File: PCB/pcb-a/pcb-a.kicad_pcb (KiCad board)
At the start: 2 copper layers, 89.4 x 42.2 mm, 29 parts, among them J1 Conn_02x05_Counter_Clockwise, J2 Conn_02x04_Counter_Clockwise, Q3 BC337, SW1 config, U1 ESP32-S2-DevKitM, U3 L7805

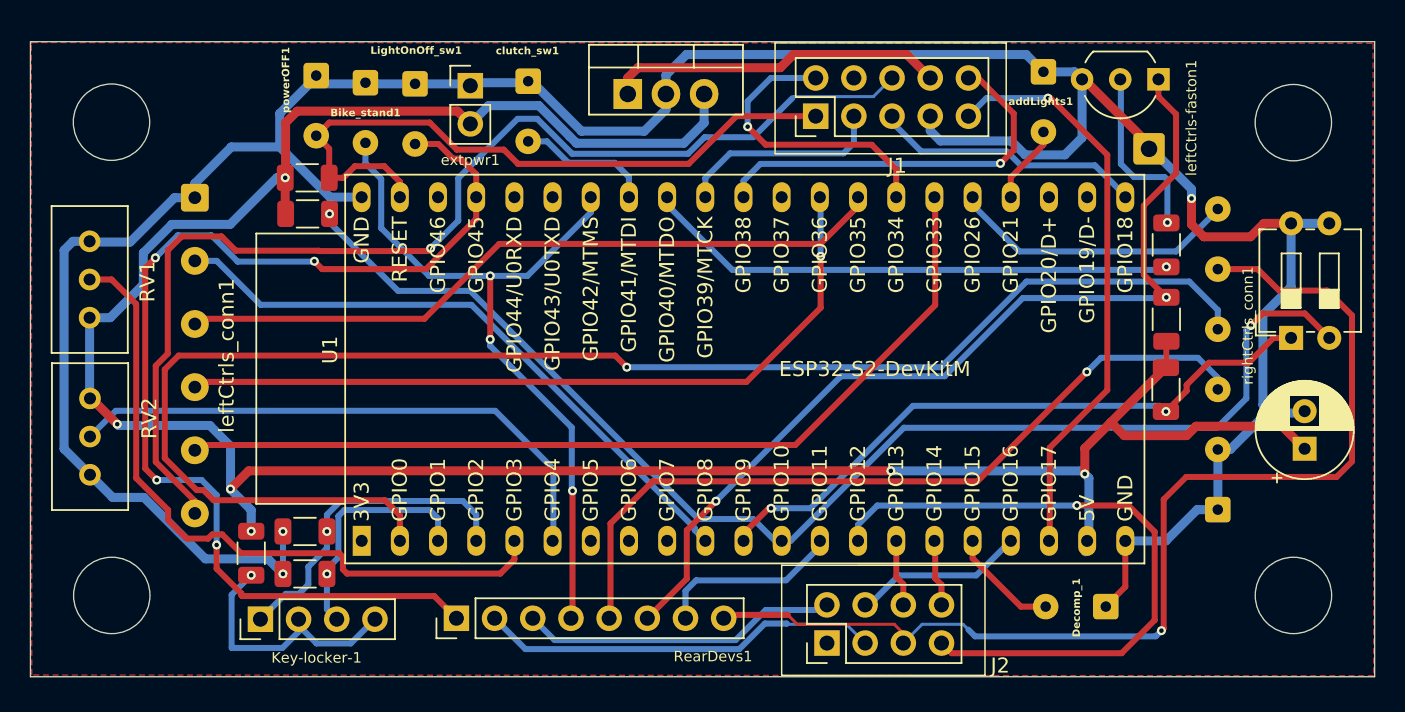
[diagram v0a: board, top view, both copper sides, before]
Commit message: Fixes
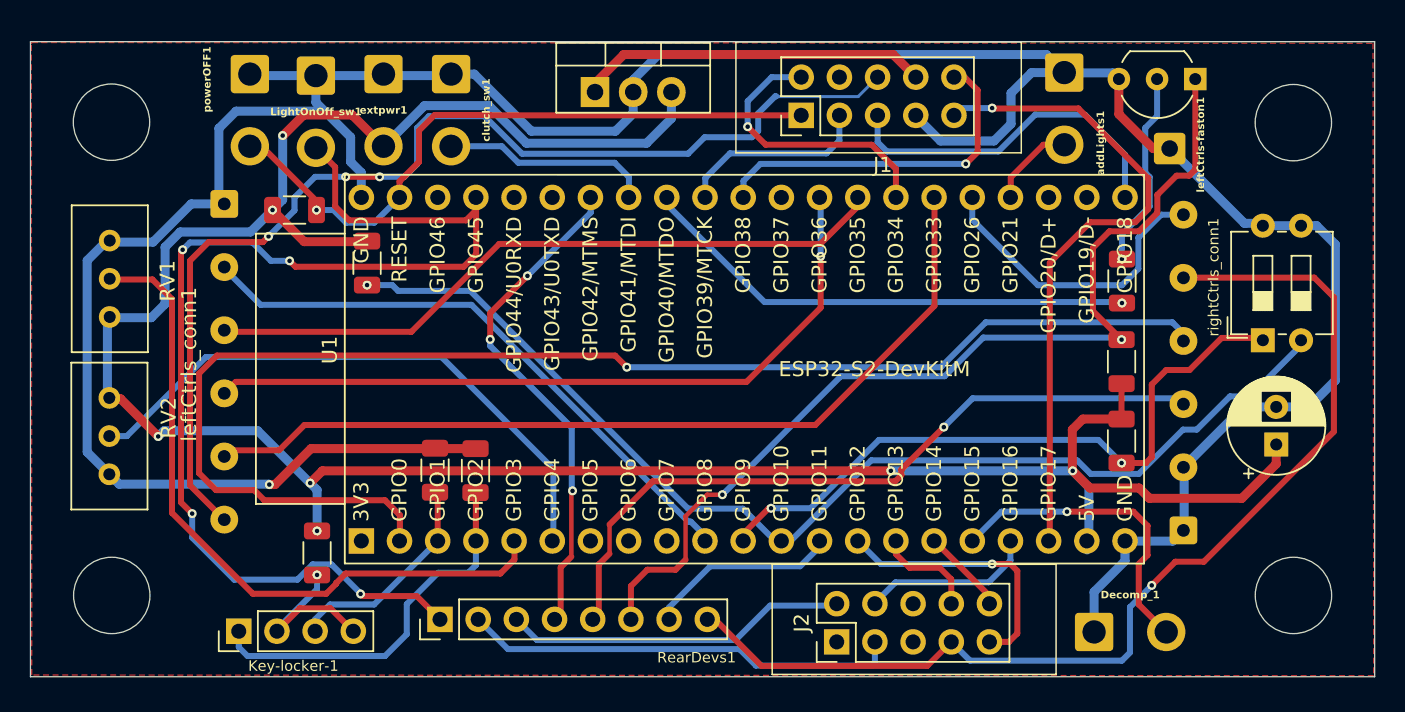
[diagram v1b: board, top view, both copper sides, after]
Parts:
- removed Bike_stand1: Conn_01x02, Connector_Wire:SolderWire-0.15sqmm_1x02_P4mm_D0.5mm_OD1.5mm
- Decomp_1, LightOnOff_sw1, addLights1, clutch_sw1, powerOFF1: footprint Connector_Wire:SolderWire-0.15sqmm_1x02_P4mm_D0.5mm_OD1.5mm -> Connector_Wire:SolderWire-0.75sqmm_1x02_P4.8mm_D1.25mm_OD2.3mm
- J2: value Conn_02x04_Counter_Clockwise -> Conn_02x05_Counter_Clockwise; footprint Connector_PinHeader_2.54mm:PinHeader_2x04_P2.54mm_Vertical -> Connector_PinHeader_2.54mm:PinHeader_2x05_P2.54mm_Vertical
- extpwr1: footprint Connector_PinHeader_2.54mm:PinHeader_1x02_P2.54mm_Vertical -> Connector_Wire:SolderWire-0.75sqmm_1x02_P4.8mm_D1.25mm_OD2.3mm
- rightCtrls_conn1: footprint Connector_Wire:SolderWire-0.15sqmm_1x06_P4mm_D0.5mm_OD1.5mm -> Connector_Wire:SolderWire-0.25sqmm_1x06_P4.2mm_D0.65mm_OD1.7mm
- moved R4 12.0 mm to (142.1, 90.7), turned to -90 degrees
- moved R3 11.1 mm to (139.4, 90.6), turned to -90 degrees
- moved LightOnOff_sw1 6.62 mm to (131.5, 64.4)
- moved extpwr1 5.83 mm to (136.0, 64.3), turned to -90 degrees
- moved clutch_sw1 5.15 mm to (140.5, 64.3)
- moved R5 5.14 mm to (134.9, 76.8), turned to -90 degrees
- moved R8 4.52 mm to (185.1, 88.7)
- moved powerOFF1 4.42 mm to (127.1, 64.3)
- moved R1 4.38 mm to (131.6, 96.1)
- moved R6 4.10 mm to (185.1, 83.4)
- moved R7 3.81 mm to (185.1, 78.0)
- moved rightCtrls_conn1 2.67 mm to (189.2, 94.6)
- moved Q3 2.45 mm to (190.0, 64.6)
- moved R2 2.30 mm to (130.1, 73.3)
- moved U3 2.18 mm to (150.1, 65.5)
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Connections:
- J2 pad 5: c_engineOFF -> unconnected-(J2-Pin_5-Pad5)
- J2 pad 6: o_engineReady -> unconnected-(J2-Pin_6-Pad6)
- J2 pad 7: o_keepAlive -> c_engineOFF
- J2 pad 8: o_neutral -> o_engineReady
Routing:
- net o_keepAlive: track 43.3 -> 17.7 mm
- net i_bykeStand: track 49.3 -> 33.7 mm
- net i_decompr: track 7.35 -> 21.5 mm, vias 0 -> 1
- net GND: track 196.3 -> 208.1 mm, vias 3 -> 1
- net Net-(U1-GPIO10/TOUCH10/ADC1_CH9/FSPICS0/FSPIIO4): track 85.4 -> 75.6 mm, vias 2 -> 1
- net i_startButton: track 100.0 -> 91.0 mm
- net Net-(Key-locker-1-Pin_2): track 17.8 -> 11.2 mm
- net o_leftArrow: track 18.0 -> 23.5 mm
- net o_upLight: track 38.6 -> 43.7 mm
- net i_clutch: track 9.02 -> 14.0 mm
- net c_rearLight: track 74.2 -> 78.9 mm
- net c_startEngine: track 62.1 -> 66.0 mm
- net c_brakeSwitch: track 52.6 -> 48.8 mm
- net i_Vx2: track 22.0 -> 25.6 mm, vias 1 -> 0
- net o_startEngine: track 36.2 -> 33.1 mm
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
